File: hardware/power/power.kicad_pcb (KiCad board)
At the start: 2 copper layers, 31.5 x 37 mm, 38 parts, among them J2 Conn_01x04_Pin, J4 Conn_01x04_Pin, P1 USB_C_Plug_USB2.0, U2 ESP32-S3-WROOM-1, U4 MCP1825S

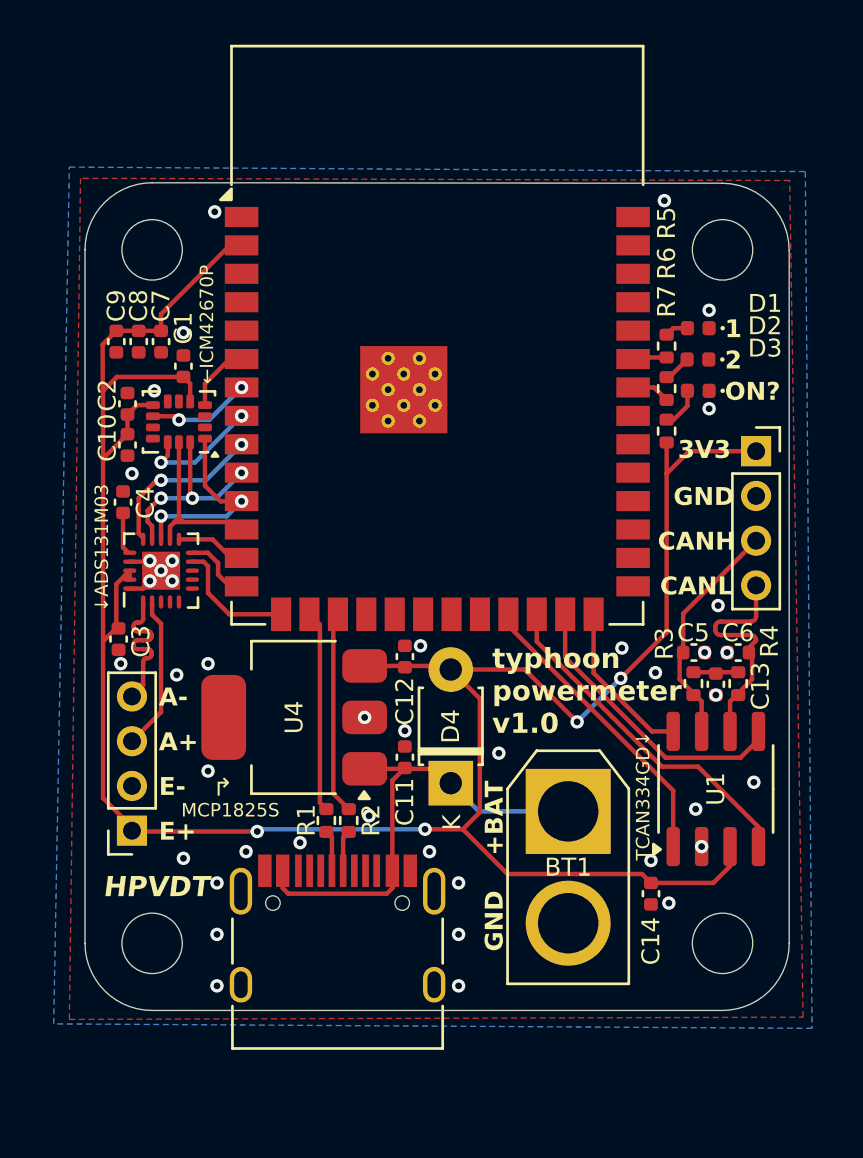
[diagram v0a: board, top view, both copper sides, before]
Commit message: major changes
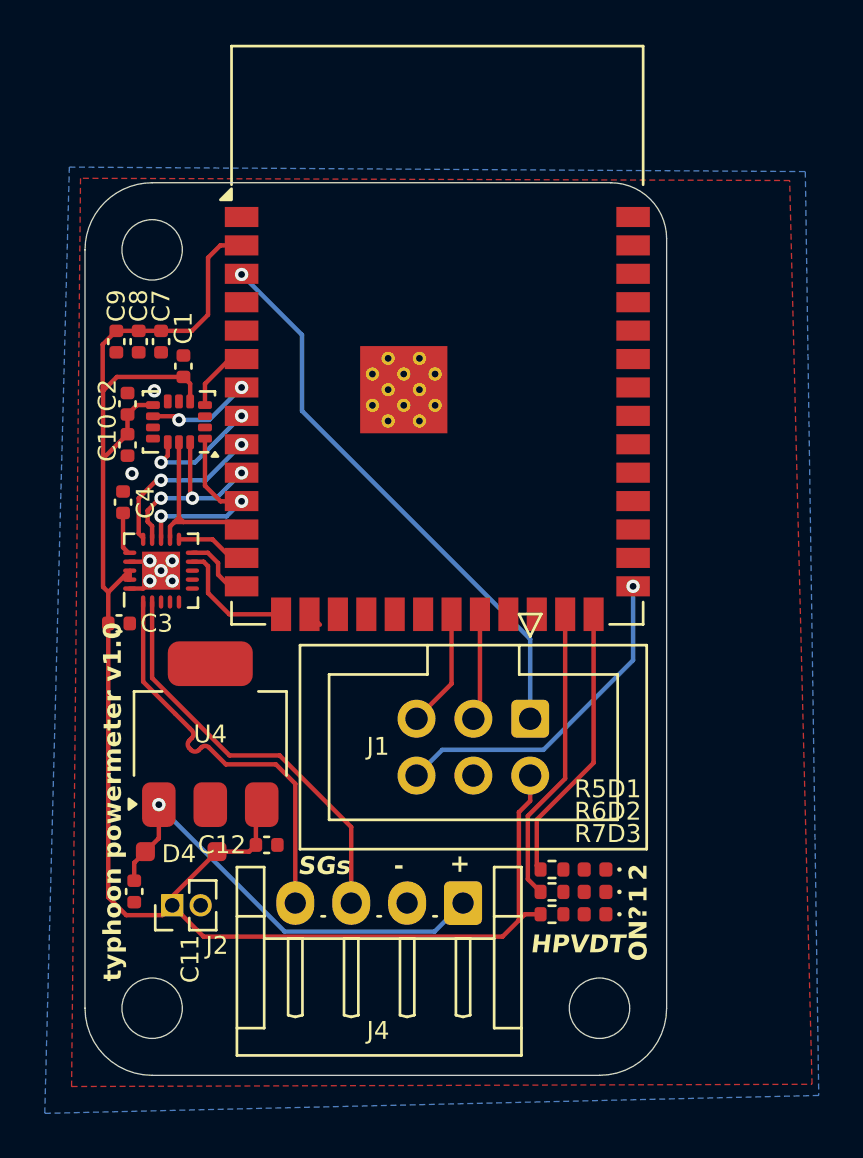
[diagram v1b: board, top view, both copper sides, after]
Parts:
- removed BT1: Battery_Cell, Connector_AMASS:AMASS_XT30U-M_1x02_P5.0mm_Vertical
- removed C13: 4.7n, Capacitor_SMD:C_0402_1005Metric
- removed C14: 100n, Capacitor_SMD:C_0402_1005Metric
- removed C5, C6: 100p, Capacitor_SMD:C_0402_1005Metric
- removed H2: M2.5, MountingHole:MountingHole_2.7mm_M2.5
- removed P1: USB_C_Plug_USB2.0, Connector_USB:USB_C_Receptacle_HRO_TYPE-C-31-M-12
- removed R1, R2: 22, Resistor_SMD:R_0402_1005Metric
- removed R3, R4: 60, Resistor_SMD:R_0402_1005Metric
- removed U1: ~, Package_SO:SO-8_3.9x4.9mm_P1.27mm
- added J1: Conn_02x03_Odd_Even, Connector_IDC:IDC-Header_2x03_P2.54mm_Vertical, F.Cu at (182.5, 80.8)
- D4: value 1N400X -> D; footprint Diode_THT:D_T-1_P5.08mm_Horizontal -> 0_myfootprints:SD103CW
- J2: value Conn_01x04_Pin -> Conn_01x02_Pin; footprint Connector_PinSocket_2.00mm:PinSocket_1x04_P2.00mm_Vertical -> Connector_PinHeader_1.27mm:PinHeader_1x02_P1.27mm_Vertical
- J4: footprint Connector_PinSocket_2.00mm:PinSocket_1x04_P2.00mm_Vertical -> Connector_JST:JST_EH_S4B-EH_1x04_P2.50mm_Horizontal
- moved J2 33.1 mm to (166.5, 89.1), turned to 90 degrees
- moved D1 24.6 mm to (185.4, 87.5)
- moved D2 24.2 mm to (185.4, 88.5)
- moved R5 24.0 mm to (183.5, 87.5), turned to 0 degrees
- moved D3 23.9 mm to (185.4, 89.5)
- moved R6 23.1 mm to (183.5, 88.5), turned to 0 degrees
- moved R7 22.2 mm to (183.5, 89.5), turned to 0 degrees
- moved J4 15.1 mm to (179.5, 89.0)
- moved C11 13.5 mm to (164.8, 88.5), turned to 90 degrees
- moved D4 12.4 mm to (166.9, 86.7), turned to 0 degrees
- moved C12 10.4 mm to (170.7, 86.4), turned to 180 degrees
- moved H4 6.22 mm to (185.6, 93.7)
- moved U4 3.82 mm to (168.2, 81.5), turned to 90 degrees
- moved H3 2.90 mm to (165.6, 93.7)
- moved C3 0.70 mm to (164.1, 76.5), turned to 180 degrees
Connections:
- ADS131M03 pad 21: (no net) -> GND
- C11 pad 2: +5V -> BATT
- D4 pad 1: +5V -> BATT
- J4 pad 1: +3V3 -> BATT
- U2 pad 16: /USB_{D}+ -> unconnected-(U2-IO46-Pad16)
- U2 pad 17: /USB_{D}- -> unconnected-(U2-IO9-Pad17)
- U2 pad 21: unconnected-(U2-IO13-Pad21) -> /RX
- U2 pad 22: unconnected-(U2-IO14-Pad22) -> /TX
- U2 pad 23: /TX -> unconnected-(U2-IO21-Pad23)
- U2 pad 24: /RX -> unconnected-(U2-IO47-Pad24)
- U2 pad 25: /SHDN_{CAN} -> /LED_{2}
- U2 pad 26: /STB_{CAN} -> /LED_{1}
- U2 pad 27: unconnected-(U2-IO0-Pad27) -> /IO0
- U2 pad 3: unconnected-(U2-EN-Pad3) -> /EN
- U2 pad 34: /LED_{2} -> unconnected-(U2-IO41-Pad34)
- U2 pad 35: /LED_{1} -> unconnected-(U2-IO42-Pad35)
- U4 pad 1: +5V -> BATT
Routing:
- net +3V3: track 110.4 -> 79.7 mm, vias 4 -> 0
- net /EN: track 0.00 -> 25.2 mm, vias 0 -> 1
- net +5V: track 21.4 -> 0.00 mm
- net BATT: track 0.00 -> 21.2 mm, vias 0 -> 1
- net /IO0: track 0.00 -> 15.1 mm, vias 0 -> 1
- net /SHDN_{CAN}: track 13.1 -> 0.00 mm
- net /LED_{2}: track 1.73 -> 13.3 mm
- net /ADS-: track 6.87 -> 18.5 mm
- net /LED_{1}: track 1.53 -> 12.5 mm
- net /ADS+: track 7.83 -> 18.4 mm
- net /CANH: track 10.3 -> 0.00 mm
- net /CANL: track 10.3 -> 0.00 mm
- net /RX: track 15.4 -> 5.32 mm
- net /USB_{D}+: track 9.24 -> 0.00 mm
- net /USB_{D}-: track 9.08 -> 0.00 mm
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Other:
- board size 31.5 x 37 mm -> 26 x 39.9 mm
- board text added: "+"
- board text added: "-"
- board text added: "SGs"
- board text removed: "- 5V USB-C - 3.7V??? LiPo?? battery - 3.3V wired"
- board text removed: "0"
- board text removed: "0 mm"
- board text removed: "0.0000 mm / 0.0000 mm"
- board text removed: "0.01 mm"
- board text removed: "0.02"
- board text removed: "0.035 mm"
- board text removed: "0.3000 mm"
- board text removed: "1.51 mm"
- board text removed: "1.6000 mm"
- board text removed: "3.3"
- board text removed: "34.6000 mm x 35.6000 mm"
- board text removed: "3V3"
- board text removed: "4.5"
- board text removed: "A+"
- board text removed: "A-"
- board text removed: "B.Cu"
- board text removed: "B.Mask"
- board text removed: "B.Paste"
- board text removed: "B.Silkscreen"
- board text removed: "BOARD CHARACTERISTICS"
- board text removed: "Board Thickness:"
- board text removed: "Board overall dimensions:"
- board text removed: "Bottom Silk Screen"
- board text removed: "Bottom Solder Mask"
- board text removed: "Bottom Solder Paste"
- board text removed: "CANH"
- board text removed: "CANL"
- board text removed: "Castellated pads:"
- board text removed: "Color"
- board text removed: "Copper Finish:"
- board text removed: "Copper Layer Count:"
- board text removed: "Dielectric"
- board text removed: "E+"
- board text removed: "E-"
- board text removed: "Edge card connectors:"
- board text removed: "Epsilon R"
- board text removed: "F.Cu"
- board text removed: "F.Mask"
- board text removed: "F.Paste"
- board text removed: "F.Silkscreen"
- board text removed: "FR4"
- board text removed: "GND"
- board text removed: "Impedance Control:"
- board text removed: "Layer Name"
- board text removed: "Loss Tangent"
- board text removed: "MCP1825S"
- board text removed: "Material"
- board text removed: "Min hole diameter:"
- board text removed: "Min track/spacing:"
- board text removed: "No"
- board text removed: "None"
- board text removed: "Not specified"
- board text removed: "Plated Board Edge:"
- board text removed: "Powered by ONE OF:"
- board text removed: "TCAN334GD↓"
- board text removed: "Thickness (mm)"
- board text removed: "Top Silk Screen"
- board text removed: "Top Solder Mask"
- board text removed: "Top Solder Paste"
- board text removed: "Type"
- board text removed: "copper"
- board text removed: "core"
- board text removed: "←ICM42670P"
- board text removed: "↓ADS131M03"
- board text removed: "↳"
